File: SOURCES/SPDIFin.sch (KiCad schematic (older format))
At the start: 1 part, among them U6 CS8422-CNZ

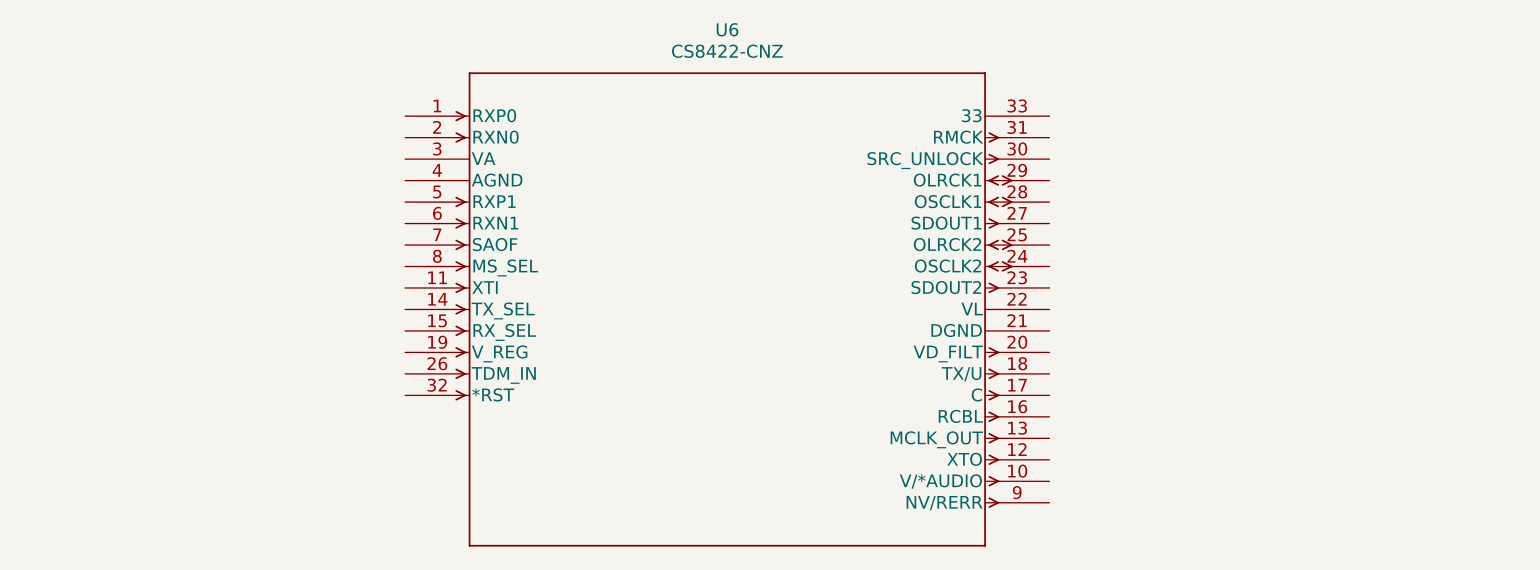
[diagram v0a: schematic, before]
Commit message: Spdif Schaltpläne
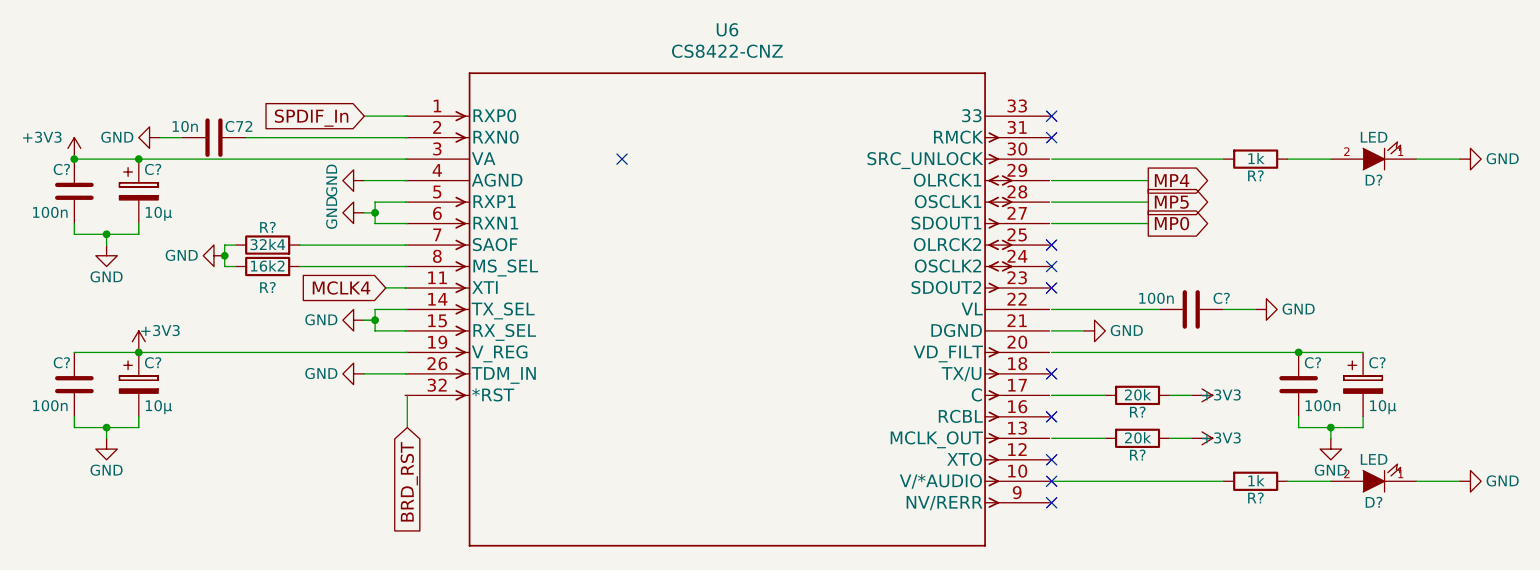
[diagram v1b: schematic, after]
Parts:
- added C72: 10n, symbol C
- added C? (x4): 100n, symbol C
- added C? (x3): 10µ, symbol CP
- added D? (x2): LED, symbol LED
- added R? (x2): 1k, symbol R
- added R? (x2): 20k, symbol R
- added R?: 32k4, symbol R
- added R?: 16k2, symbol R
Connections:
- net labels added: +3V3, BRD_RST, GND, MCLK4, MP0, MP4, MP5, SPDIF_In
- wire segments 0 -> 51
- no-connect marks 0 -> 11
